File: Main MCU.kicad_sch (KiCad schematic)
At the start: 48 parts, among them J10 Conn_01x02_Pin, J9 Conn_01x06_Pin, U1 STM32F407VGTx, U5 MCP1825S-3302E/EB

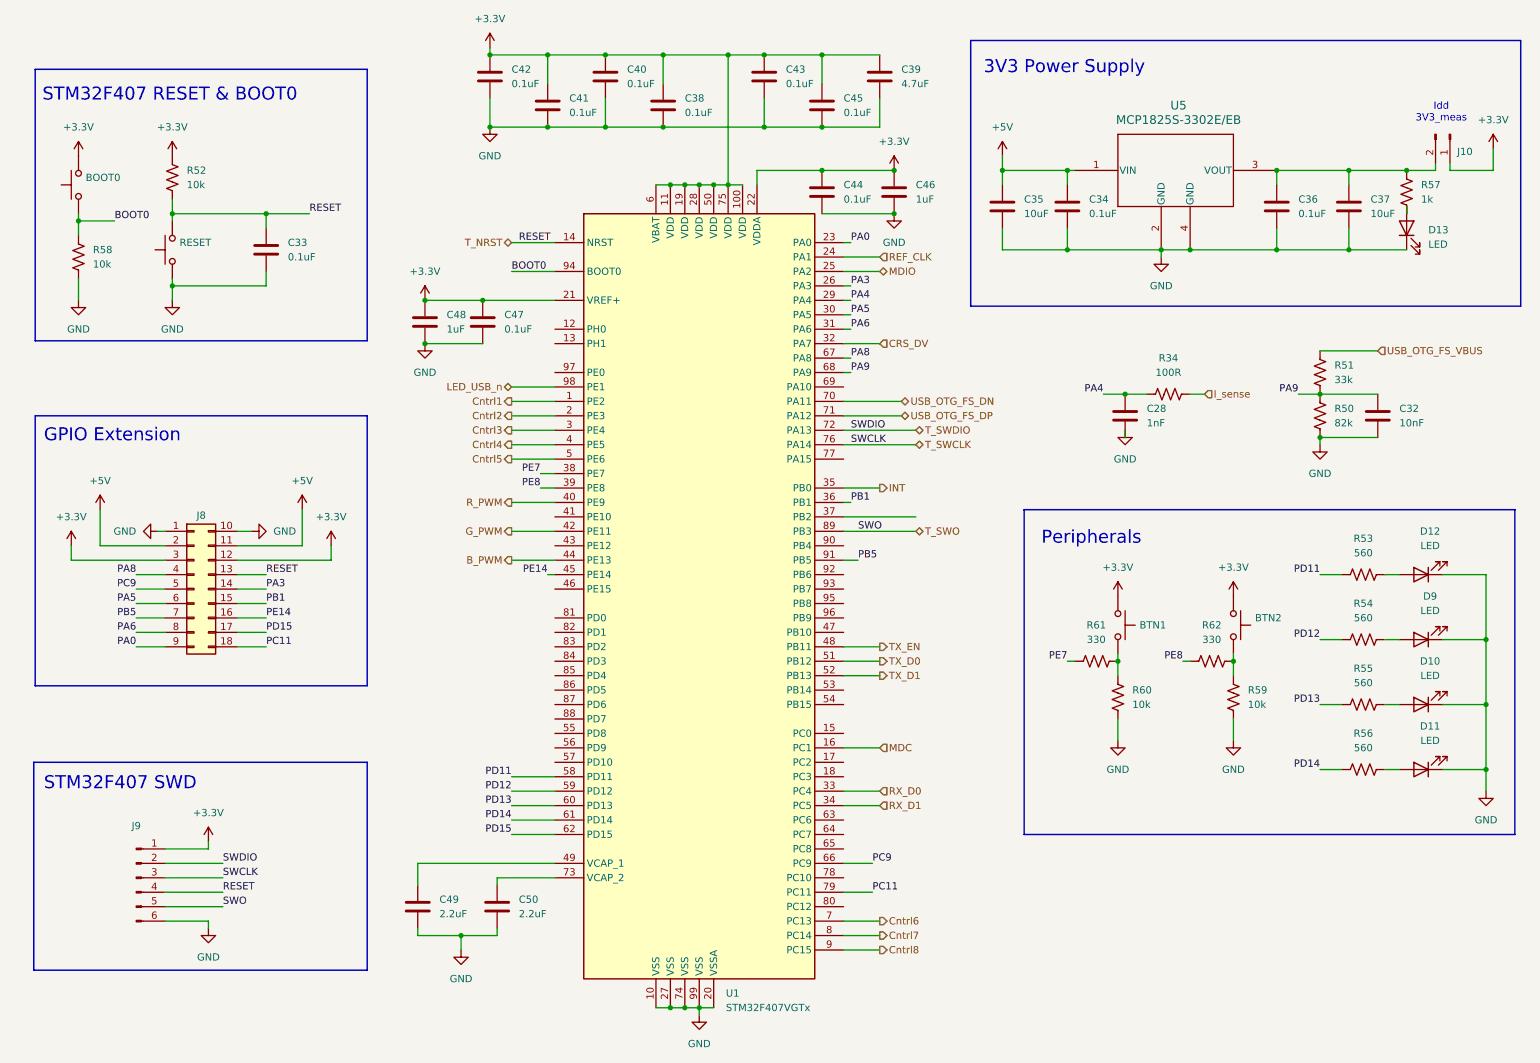
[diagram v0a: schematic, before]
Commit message: update
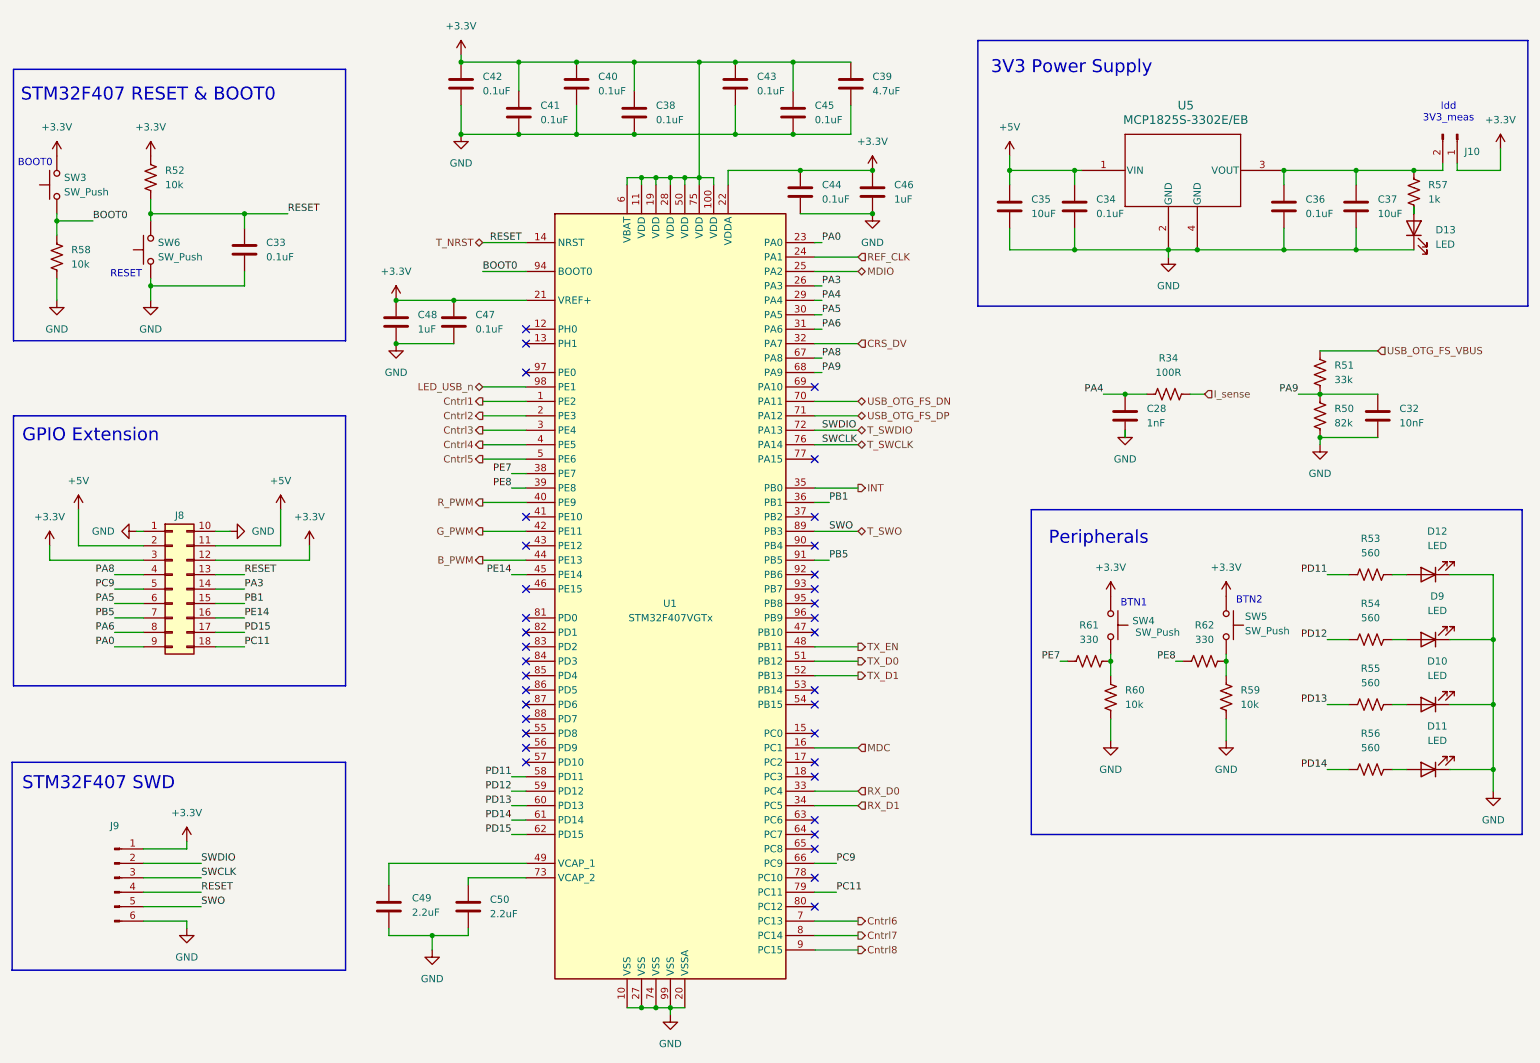
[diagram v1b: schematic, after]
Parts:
- C32: footprint Capacitor_SMD:C_0603_1608Metric -> Capacitor_SMD:C_0402_1005Metric; MPN (none) -> GRM155R71E103KA01D; Manufacturer (none) -> Murata Electronics
- D10, D11, D12, D13, D9: footprint (none) -> LED_SMD:LED_0805_2012Metric
- SW3: renamed from BOOT0; value ~ -> SW_Push
- SW4: renamed from BTN1; value ~ -> SW_Push
- SW5: renamed from BTN2; value ~ -> SW_Push
- SW6: renamed from RESET; value RESET -> SW_Push
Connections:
- no-connect marks 0 -> 36
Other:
- note added: "BOOT0"
- note added: "BTN1"
- note added: "BTN2"
- note added: "RESET"
- moved on the sheet: C33, C34, C35, C36, C37, C38, C39, C40, C41, C42, C43, C44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
